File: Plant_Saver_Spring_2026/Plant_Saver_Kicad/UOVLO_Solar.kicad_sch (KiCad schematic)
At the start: 10 parts, among them Q11 ISP12DP06NMXTSA1, Q12 G09P02L, U16 MCP6547T_I_MS

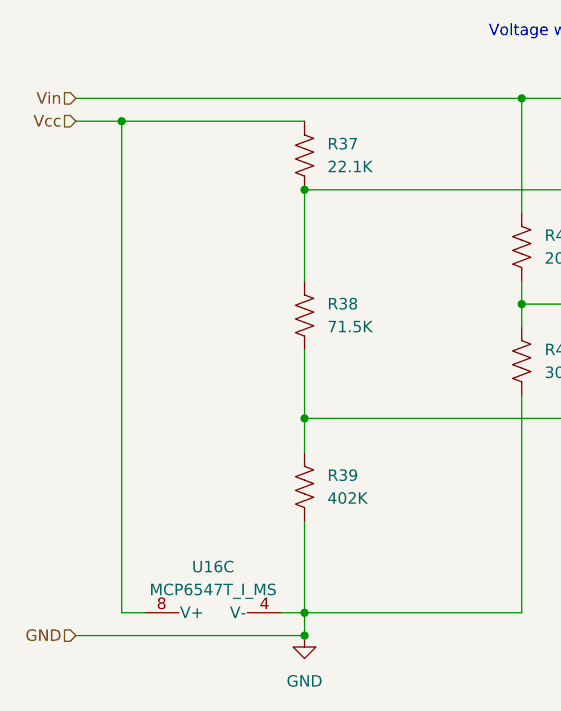
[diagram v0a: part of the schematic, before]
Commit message: Resub from last
I forgot to save some of my changes from my last push
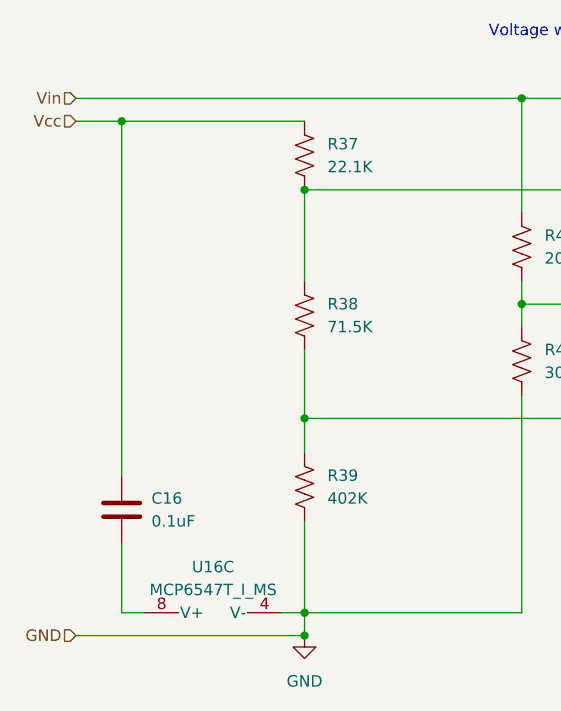
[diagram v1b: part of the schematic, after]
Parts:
- added C16: 0.1uF, Capacitor_THT:C_Disc_D4.7mm_W2.5mm_P5.00mm, symbol Device:C
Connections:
- net Vcc: now also C16.1; no longer U16.8 (V+)
- new net: C16.2, U16.8 (V+)
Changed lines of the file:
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@@
 	(wire
 		(pts
-			(xy 93.98 71.12) (xy 93.98 125.73)
+			(xy 93.98 71.12) (xy 93.98 110.49)
 		)
 		(stroke
@@
 		(pts
 			(xy 138.43 93.98) (xy 138.43 91.44)
+		)
+		(stroke
+			(width 0)
+			(type default)
+		)
+	)
+	(wire
+		(pts
+			(xy 93.98 118.11) (xy 93.98 125.73)
 		)
 		(stroke
@@
 					(unit 1)
 				)
+			)
+		)
+	)
+	(symbol
+		(lib_id "Device:C")
+		(at 93.98 114.3 0)
+		(unit 1)
+		(exclude_from_sim no)
+		(in_bom yes)
+		(on_board yes)
+		(dnp no)
+		(property "Reference" "C16"
+			(at 97.282 113.03 0)
+			(effects
+				(font
+					(size 1.27 1.27)
+				)
+				(justify left)
+			)
+		)
+		(property "Value" "0.1uF"
+			(at 97.282 115.57 0)
+			(effects
+				(font
+					(size 1.27 1.27)
+				)
+				(justify left)
+			)
+		)
+		(property "Footprint" "Capacitor_THT:C_Disc_D4.7mm_W2.5mm_P5.00mm"
+			(at 94.9452 118.11 0)
+			(effects
+				(font
+					(size 1.27 1.27)
+				)
+				(hide yes)
+			)
+		)
+		(property "Datasheet" "~"
+			(at 93.98 114.3 0)
+			(effects
+				(font
+					(size 1.27 1.27)
+				)
+				(hide yes)
+			)
+		)
+		(property "Description" "Unpolarized capacitor"
+			(at 93.98 114.3 0)
+			(effects
+				(font
+					(size 1.27 1.27)
+				)
+				(hide yes)
+			)
+		)
+		(pin "1"
+		)
+		(pin "2"
+		)
+		(instances
+			(project "Plant_Saver_Kicad"
+				(path "/7f244634-d37a-4ff0-ba36-8027330ab1bd/c1b5c94f-5fb5-4e2b-895b-5d171c372d7d/9fa29de7-25a7-4316-bbea-8ab2651dedf4"
+					(reference "C16")
+					(unit 1)
+				)
